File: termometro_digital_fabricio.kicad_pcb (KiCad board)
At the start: 2 copper layers, 19 parts, among them SW1 SW_Push, U1 MT3608, U3 LM35-LP, U4 ICL7107CPL

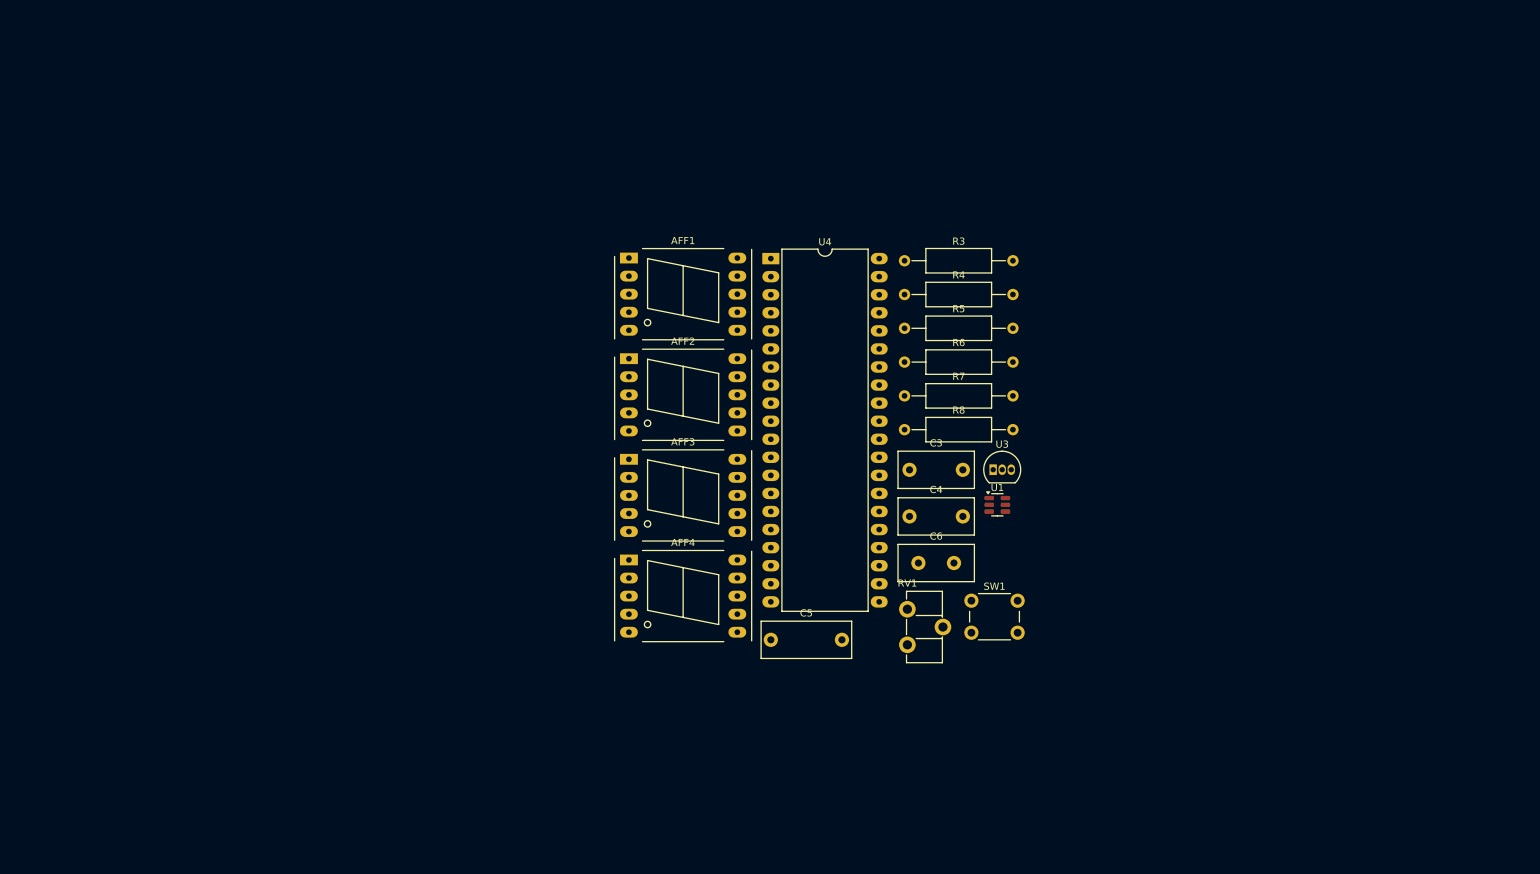
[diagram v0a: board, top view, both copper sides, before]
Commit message: Uploading files
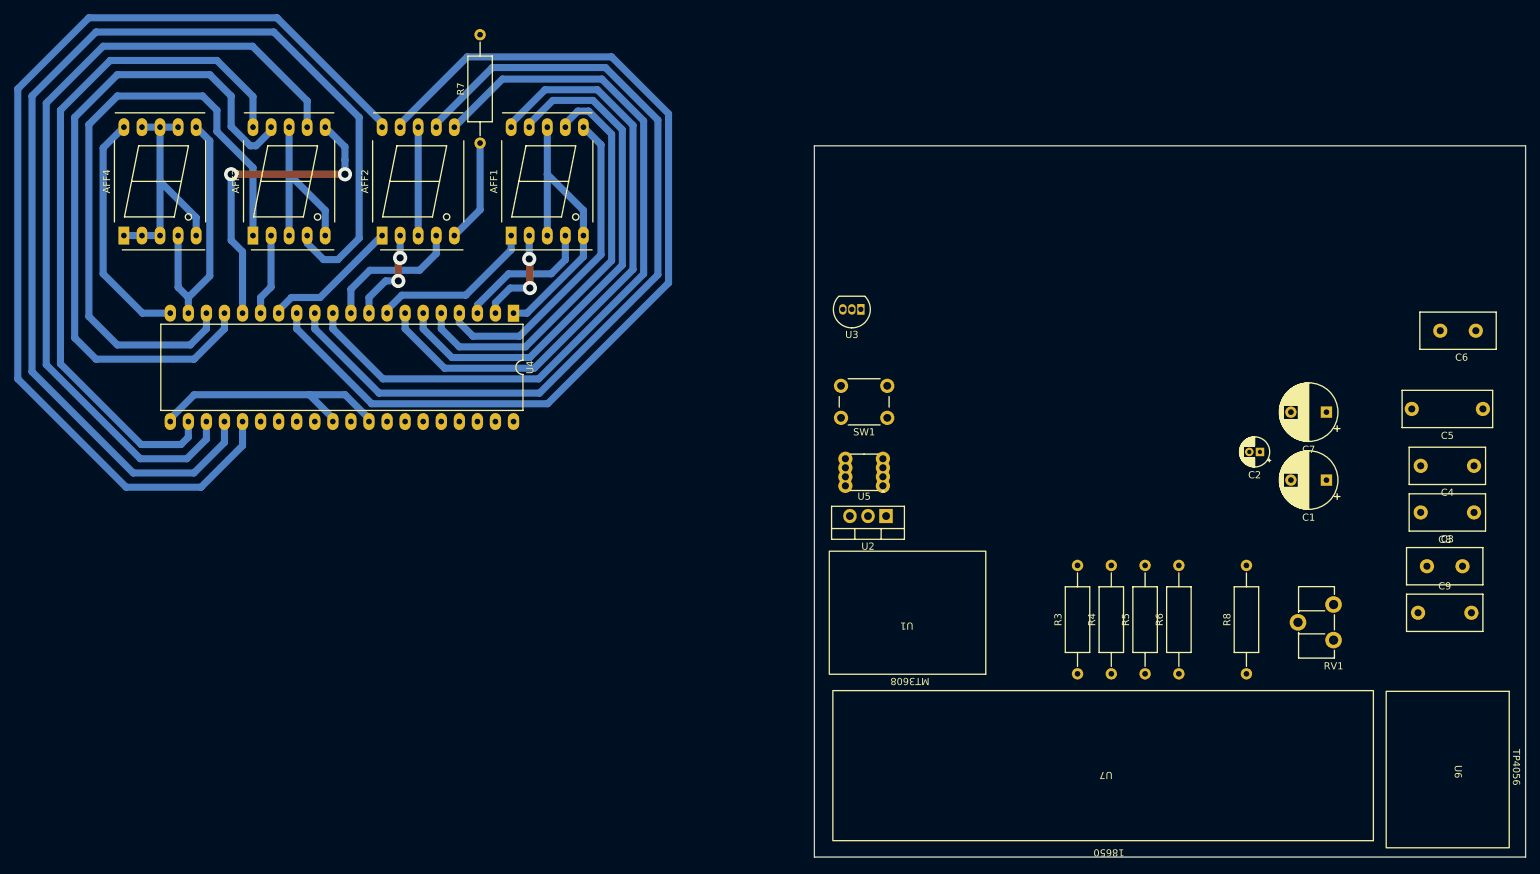
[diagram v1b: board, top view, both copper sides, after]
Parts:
- added C1: C_Polarized, Capacitor_THT:CP_Radial_D8.0mm_P5.00mm, F.Cu at (203.0, 93.0)
- added C2: 1uF, Capacitor_THT:CP_Radial_D4.0mm_P1.50mm, F.Cu at (193.6, 89.0)
- added C7: C_Polarized, Capacitor_THT:CP_Radial_D8.0mm_P5.00mm, F.Cu at (203.0, 83.5)
- added C8: 1nF, Capacitor_THT:C_Disc_D10.5mm_W5.0mm_P5.00mm, F.Cu at (217.1, 105.1)
- added C9: 0.01uF, Capacitor_THT:C_Disc_D10.5mm_W5.0mm_P7.50mm, F.Cu at (215.9, 111.7)
- added U2: L7805, Package_TO_SOT_THT:TO-220-3_Vertical, F.Cu at (141.1, 98.1)
- added U5: ICL7660, Library:SOIC-8, F.Cu at (138.0, 91.9)
- added U6: ~, Library:TP4056, F.Cu at (221.0, 134.0)
- added U7: 18650, Library:18650, F.Cu at (172.0, 134.0)
- R5: value 100k -> 24K
- U1: footprint Package_TO_SOT_SMD:SOT-23-6 -> Library:MT3608
- moved C5 105.3 mm to (225.0, 83.0), turned to 180 degrees
- moved C6 84.9 mm to (224.0, 72.0), turned to 180 degrees
- moved AFF4 84.4 mm to (33.9, 58.6), turned to 90 degrees
- moved C4 79.7 mm to (223.8, 91.0), turned to 180 degrees
- moved C3 79.6 mm to (223.8, 97.5), turned to 180 degrees
- moved R7 69.5 mm to (84.0, 45.6), turned to 90 degrees
- moved R3 63.0 mm to (168.0, 120.2), turned to 90 degrees
- moved AFF3 61.5 mm to (52.1, 58.6), turned to 90 degrees
- moved R4 60.7 mm to (172.8, 120.2), turned to 90 degrees
- moved RV1 60.1 mm to (204.0, 115.5), turned to 180 degrees
- moved R5 59.2 mm to (177.5, 120.2), turned to 90 degrees
- moved R8 59.1 mm to (191.8, 120.2), turned to 90 degrees
- moved R6 58.4 mm to (182.2, 120.2), turned to 90 degrees
- moved AFF2 38.8 mm to (70.2, 58.6), turned to 90 degrees
- moved U4 37.0 mm to (88.7, 69.5), turned to -90 degrees
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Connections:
- R7 pad 2: GND -> Net-(U4-V-)
- U4 pad 26: VEE -> Net-(U4-V-)
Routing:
- net Net-(AFF3-c): track 0.00 -> 158.7 mm
- net Net-(AFF2-g): track 0.00 -> 146.6 mm
- net Net-(AFF2-f): track 0.00 -> 135.2 mm
- net Net-(AFF2-a): track 0.00 -> 120.8 mm
- net VCC: track 0.00 -> 118.4 mm
- net Net-(AFF3-a): track 0.00 -> 115.3 mm
- net Net-(AFF2-b): track 0.00 -> 108.3 mm
- net Net-(AFF3-g): track 0.00 -> 97.3 mm
- net Net-(AFF3-f): track 0.00 -> 95.4 mm
- net Net-(AFF3-e): track 0.00 -> 88.5 mm
- net Net-(AFF1-g): track 0.00 -> 84.2 mm
- net Net-(AFF1-f): track 0.00 -> 72.9 mm
- net Net-(AFF1-a): track 0.00 -> 59.1 mm
- net Net-(AFF1-b): track 0.00 -> 45.7 mm
- net Net-(AFF3-b): track 0.00 -> 44.0 mm, vias 0 -> 2
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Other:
- board outline added: 100 x 100 mm
